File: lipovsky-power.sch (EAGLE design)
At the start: 101 parts, among them J1 M04-929J, J2 M04-929J, J3 M04-929J, J4 M04-929J, Q1 NMOS30V_30A, Q11 NMOS40V_10A, Q12 NMOS40V_10A, Q14 NMOS40V_10A, Q15 NMOS40V_10A, Q16 NMOS40V_10A, Q18 NMOS40V_10A, Q2 2NMOS30V_0.1A, Q21 PMOS30V_11A, Q22 PMOS30V_11A, Q23 NMOS40V_10A, Q24 NMOS40V_10A, Q25 PMOS30V_11A, Q26 PMOS30V_11A, Q27 NMOS40V_10A, Q28 NMOS40V_10A, Q3 2PMOS50V_0.17A, Q31 PMOS30V_11A, Q32 PMOS30V_11A, Q33 PMOS30V_11A, Q34 PMOS30V_11A, Q35 PMOS30V_11A, Q36 PMOS30V_11A, Q37 PMOS30V_11A, Q38 PMOS30V_11A, Q4 2PMOS50V_0.17A, Q41 PMOS30V_11A, Q42 PMOS30V_11A, Q43 PMOS30V_11A, Q44 PMOS30V_11A, Q45 PMOS30V_11A, Q46 PMOS30V_11A, Q47 PMOS30V_11A, Q48 PMOS30V_11A, Q5 2NMOS30V_0.1A, Q51 PMOS30V_11A, Q52 PMOS30V_11A, Q53 PMOS30V_11A, Q54 PMOS30V_11A, Q55 PMOS30V_11A, Q56 PMOS30V_11A, Q57 PMOS30V_11A, Q58 PMOS30V_11A, Q62 PMOS30V_11A, Q64 PMOS30V_11A, Q66 PMOS30V_11A, Q68 PMOS30V_11A, T1 TFORM_4_4311_4A4, U1 DG508BEN-T1-GE4, U2 DG508BEN-T1-GE4, U3 74HC595, U4 LTC3805-5IDD, U5 TC1240A, U6 AR30N60PPA-13

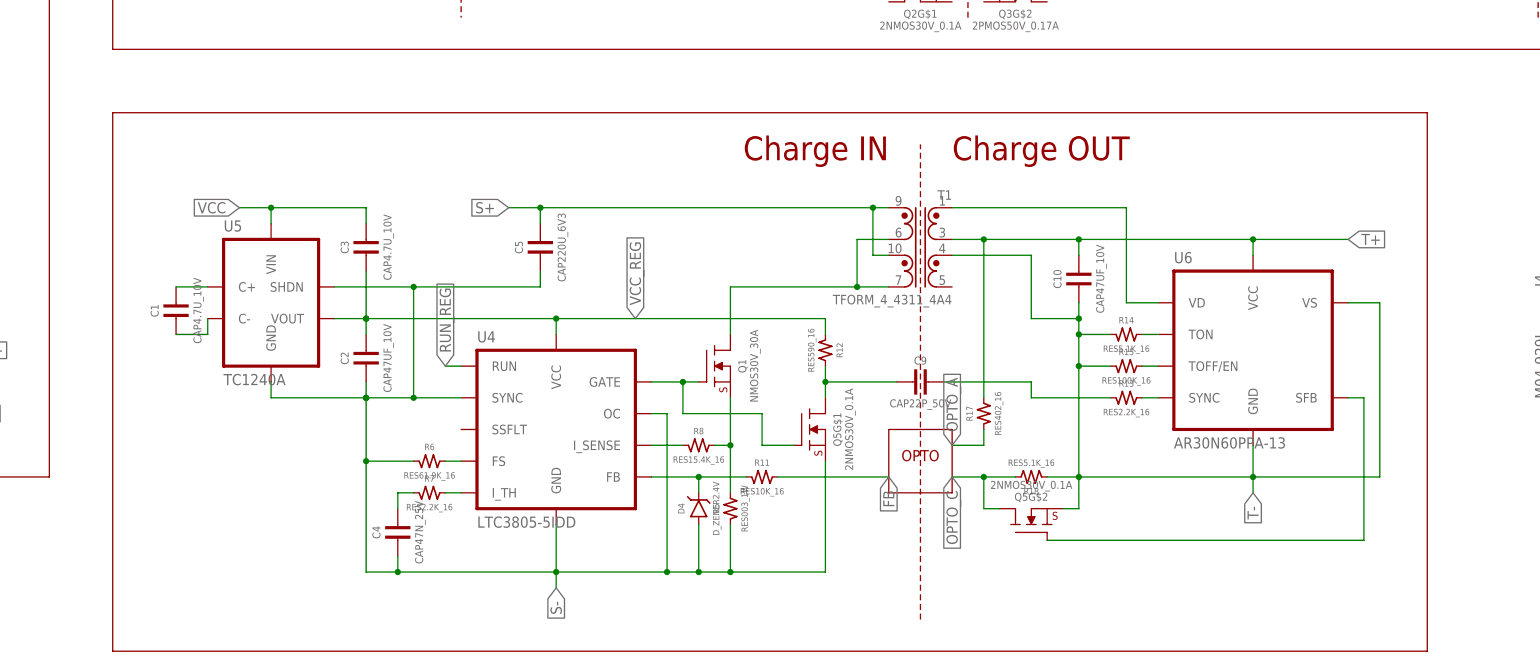
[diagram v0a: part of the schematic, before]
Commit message: .
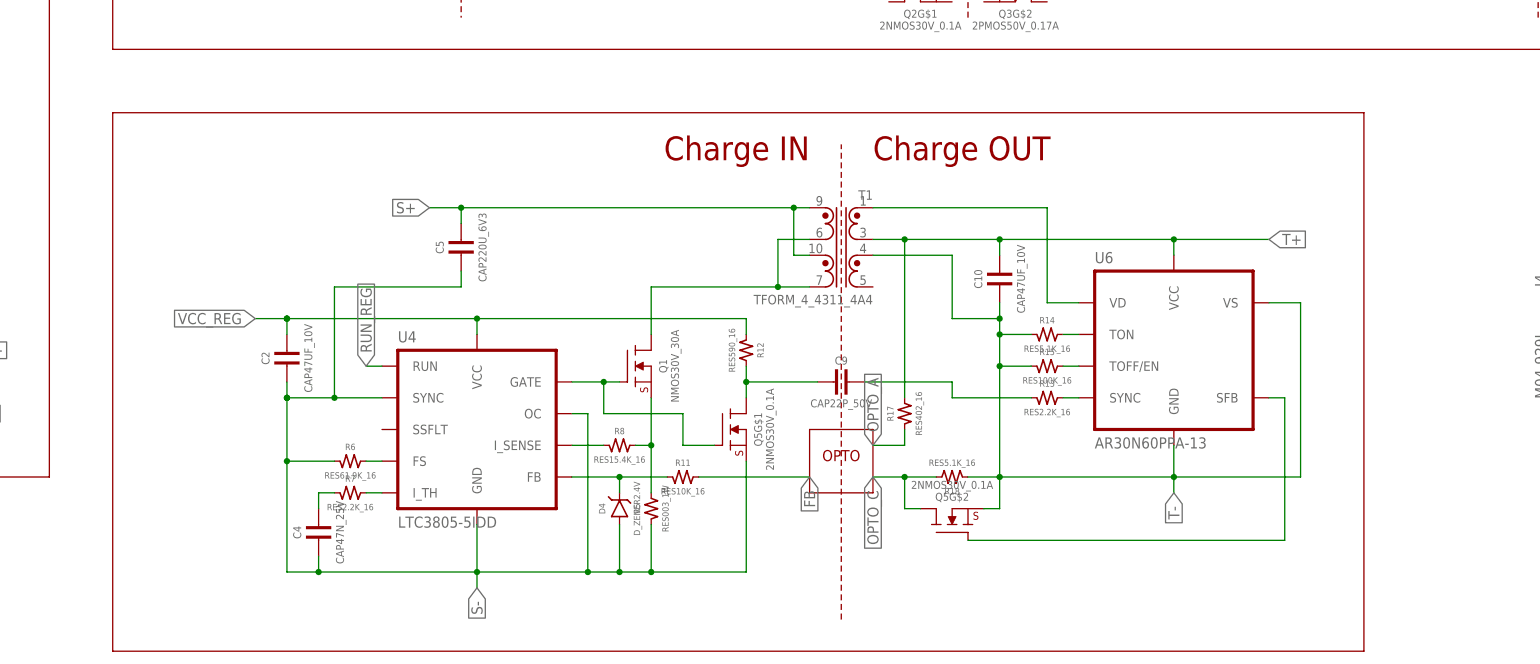
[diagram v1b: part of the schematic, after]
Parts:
- removed C1, C3: CAP4.7U_10V, dubec:CAP4.7U_10V
- removed U5: TC1240A, dubec:TC1240A
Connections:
- removed net N$8: C1.2, U5.C+
- removed net N$9: C1.1, U5.C-
- net S-: no longer U5.GND, U5.SHDN
- net VCC: no longer C3.2, U5.VIN
- net VCC_REG: no longer C3.1, U5.VOUT
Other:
- moved on the sheet: C10, C2, C4, C5, C9, D4, Q1, Q5G$1, Q5G$2, R11, R12, R13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

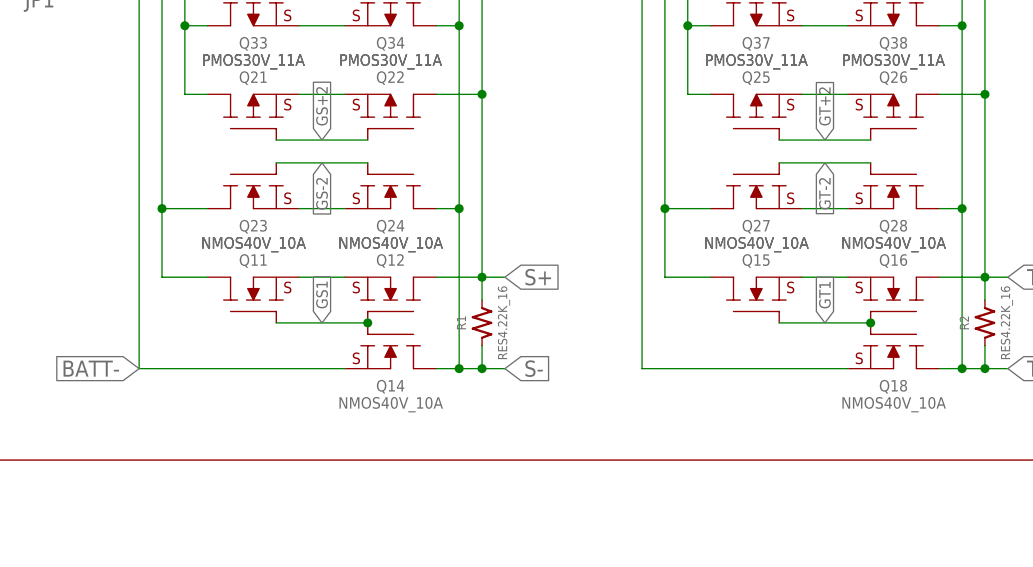
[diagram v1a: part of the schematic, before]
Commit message: .
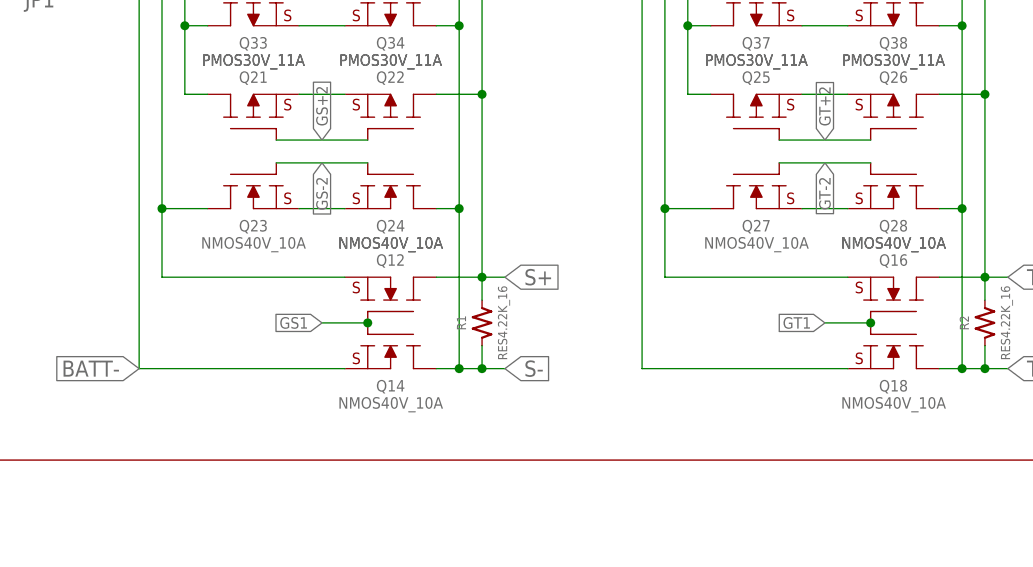
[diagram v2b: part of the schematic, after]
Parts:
- removed Q11, Q15: NMOS40V_10A, dubec:NMOS40V_10A
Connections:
- removed net SS+1: Q11.S, Q12.S
- removed net ST+1: Q15.S, Q16.S
- net C1: now also Q12.S, Q16.S; no longer Q11.D, Q15.D
- net GS1: no longer Q11.G
- net GT1: no longer Q15.G
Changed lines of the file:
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@@
 <part name="R2" library="dubec" deviceset="RES" device="4.22K_16"/>
 <part name="T1" library="dubec" deviceset="TFORM_4_4" device="311_4A4"/>
-<part name="Q11" library="dubec" deviceset="NMOS" device="40V_10A"/>
 <part name="Q12" library="dubec" deviceset="NMOS" device="40V_10A"/>
 <part name="Q23" library="dubec" deviceset="NMOS" device="40V_10A"/>
@@
 <part name="Q27" library="dubec" deviceset="NMOS" device="40V_10A"/>
 <part name="Q28" library="dubec" deviceset="NMOS" device="40V_10A"/>
-<part name="Q15" library="dubec" deviceset="NMOS" device="40V_10A"/>
 <part name="Q16" library="dubec" deviceset="NMOS" device="40V_10A"/>
 <part name="RGT6" library="dubec" deviceset="RES" device="100K_16"/>
@@
 <instance part="R2" gate="G$1" x="-20.32" y="-48.26" rot="R90"/>
 <instance part="T1" gate="G$1" x="121.92" y="-27.94" rot="MR0"/>
-<instance part="Q11" gate="G$1" x="-101.6" y="-43.18" rot="R90"/>
 <instance part="Q12" gate="G$1" x="-86.36" y="-43.18" rot="MR90"/>
 <instance part="Q23" gate="G$1" x="-101.6" y="-35.56" rot="MR270"/>
@@
 <instance part="Q27" gate="G$1" x="-45.72" y="-35.56" rot="MR270"/>
 <instance part="Q28" gate="G$1" x="-30.48" y="-35.56" rot="R270"/>
-<instance part="Q15" gate="G$1" x="-45.72" y="-43.18" rot="R90"/>
 <instance part="Q16" gate="G$1" x="-30.48" y="-43.18" rot="MR90"/>
 <instance part="RGT6" gate="G$1" x="167.64" y="71.12"/>
@@
 <wire x1="-111.76" y1="-35.56" x2="-111.76" y2="-43.18" width="0.1524" layer="91"/>
 <wire x1="-111.76" y1="-5.08" x2="-119.38" y2="-5.08" width="0.1524" layer="91"/>
-<pinref part="Q11" gate="G$1" pin="D"/>
-<wire x1="-106.68" y1="-43.18" x2="-111.76" y2="-43.18" width="0.1524" layer="91"/>
 <pinref part="Q23" gate="G$1" pin="D"/>
 <wire x1="-111.76" y1="-35.56" x2="-106.68" y2="-35.56" width="0.1524" layer="91"/>
 <junction x="-111.76" y="-35.56"/>
+<pinref part="Q12" gate="G$1" pin="S"/>
+<wire x1="-111.76" y1="-43.18" x2="-91.44" y2="-43.18" width="0.1524" layer="91"/>
 </segment>
 <segment>
@@
 <wire x1="-55.88" y1="-35.56" x2="-55.88" y2="-43.18" width="0.1524" layer="91"/>
 <junction x="-55.88" y="-35.56"/>
-<wire x1="-55.88" y1="-43.18" x2="-50.8" y2="-43.18" width="0.1524" layer="91"/>
 <label x="-63.5" y="-5.08" size="1.27" layer="95" rot="R180" xref="yes"/>
 <pinref part="Q27" gate="G$1" pin="D"/>
-<pinref part="Q15" gate="G$1" pin="D"/>
+<pinref part="Q16" gate="G$1" pin="S"/>
+<wire x1="-55.88" y1="-43.18" x2="-35.56" y2="-43.18" width="0.1524" layer="91"/>
 </segment>
 </net>
@@
 <pinref part="Q14" gate="G$1" pin="G"/>
 <pinref part="Q12" gate="G$1" pin="G"/>
-<label x="-93.98" y="-48.26" size="1.27" layer="95" rot="R90" xref="yes"/>
-<pinref part="Q11" gate="G$1" pin="G"/>
-<wire x1="-99.06" y1="-48.26" x2="-88.9" y2="-48.26" width="0.1524" layer="91"/>
+<label x="-93.98" y="-48.26" size="1.27" layer="95" rot="R180" xref="yes"/>
+<wire x1="-93.98" y1="-48.26" x2="-88.9" y2="-48.26" width="0.1524" layer="91"/>
 <junction x="-88.9" y="-48.26"/>
 </segment>
@@
 </segment>
 </net>
-<net name="SS+1" class="0">
-<segment>
-<pinref part="Q12" gate="G$1" pin="S"/>
-<pinref part="Q11" gate="G$1" pin="S"/>
-<wire x1="-96.52" y1="-43.18" x2="-91.44" y2="-43.18" width="0.1524" layer="91"/>
-</segment>
-</net>
 <net name="C4+" class="0">
 <segment>
@@
 <pinref part="Q16" gate="G$1" pin="G"/>
 <pinref part="Q18" gate="G$1" pin="G"/>
-<pinref part="Q15" gate="G$1" pin="G"/>
-<wire x1="-33.02" y1="-48.26" x2="-43.18" y2="-48.26" width="0.1524" layer="91"/>
+<wire x1="-33.02" y1="-48.26" x2="-38.1" y2="-48.26" width="0.1524" layer="91"/>
 <junction x="-33.02" y="-48.26"/>
-<label x="-38.1" y="-48.26" size="1.27" layer="95" rot="R90" xref="yes"/>
+<label x="-38.1" y="-48.26" size="1.27" layer="95" rot="R180" xref="yes"/>
 </segment>
 <segment>
@@
 </segment>
 </net>
-<net name="ST+1" class="0">
-<segment>
-<pinref part="Q15" gate="G$1" pin="S"/>
-<pinref part="Q16" gate="G$1" pin="S"/>
-<wire x1="-40.64" y1="-43.18" x2="-35.56" y2="-43.18" width="0.1524" layer="91"/>
-</segment>
-</net>
